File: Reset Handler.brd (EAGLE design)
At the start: 67 x 39.4 mm, 13 parts, among them IC1 NE555P, T1 2N222A

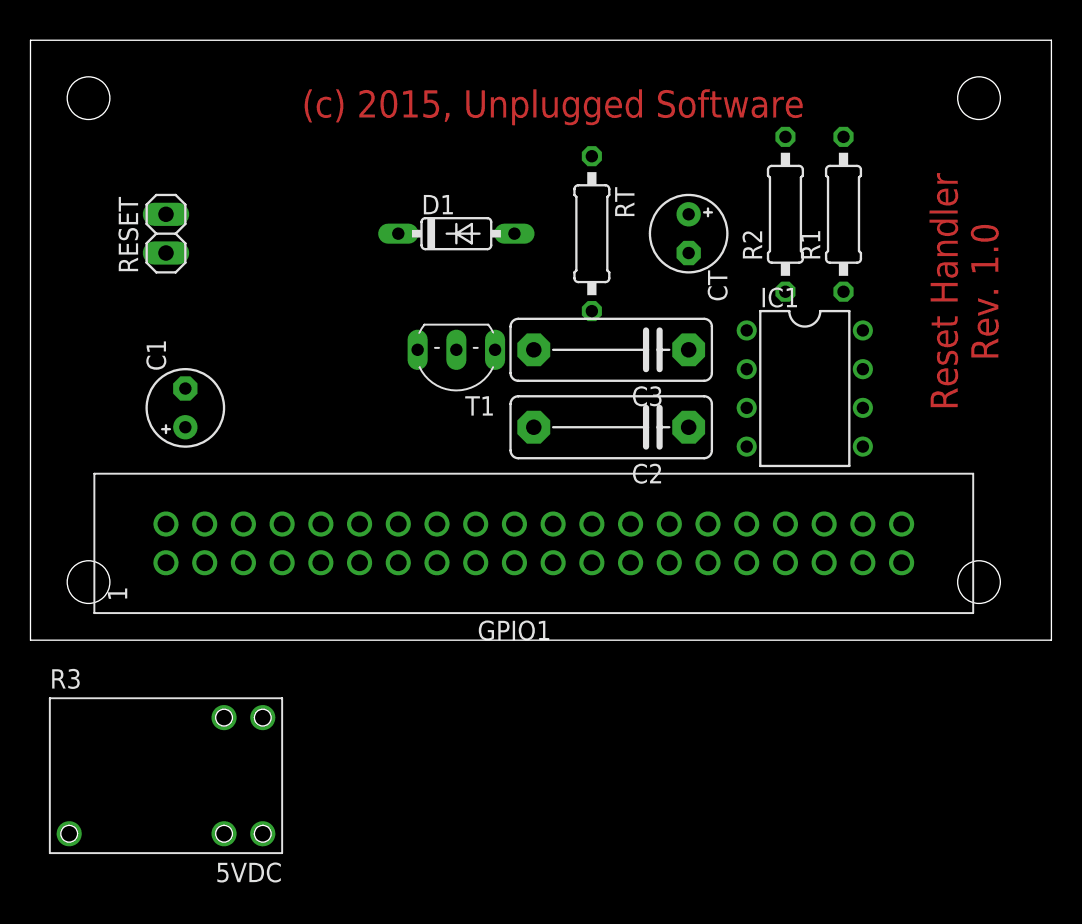
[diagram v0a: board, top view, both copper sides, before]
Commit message: Finished Reset Handler board.
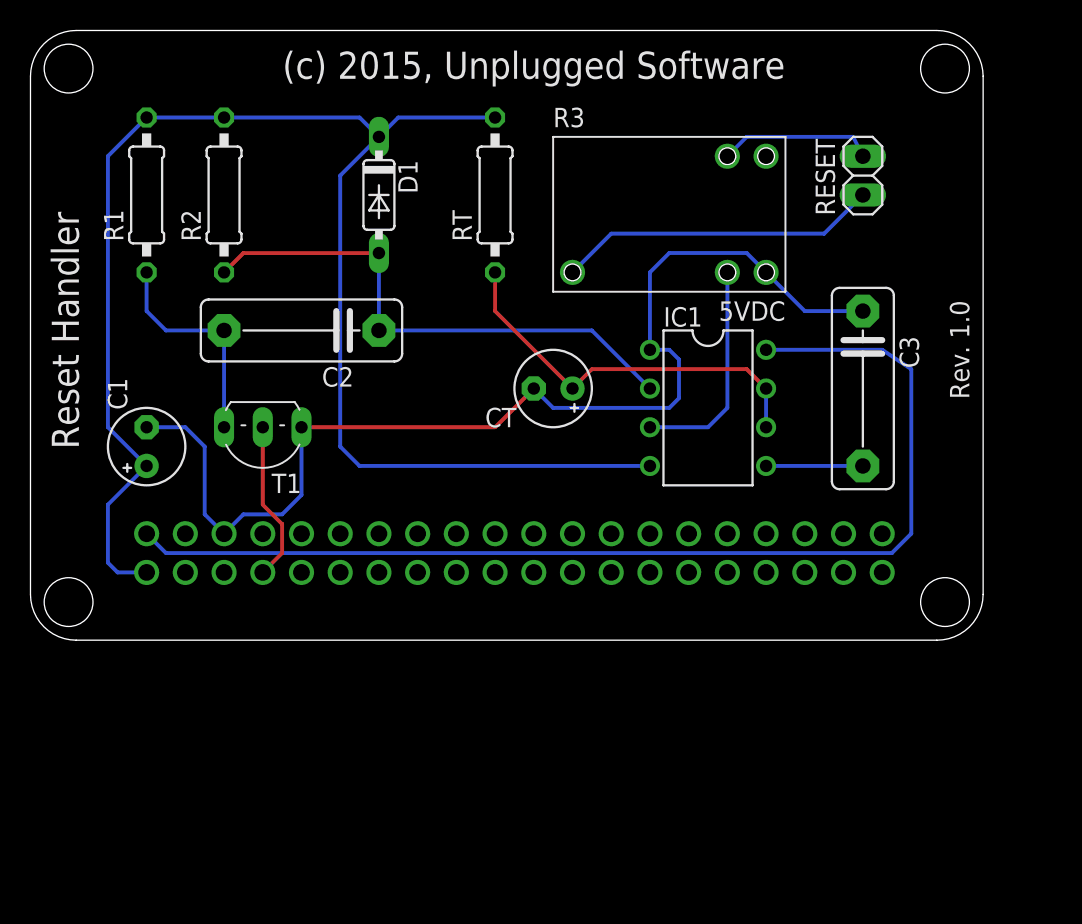
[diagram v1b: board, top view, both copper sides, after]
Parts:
- D1: value 1N4148DO35-7 -> 1N4148
- GPIO1: value RPI_GPIOUPPER -> RPI_GPIO_MALE_OPEN; device connectors:RPI_GPIO_MALE -> connectors:RPI_GPIO_FEMALE_TOP
- moved R3 49.5 mm to (41.9, 27.9)
- moved RESET 45.9 mm to (54.6, 30.5)
- moved R1 45.7 mm to (7.62, 29.2)
- moved R2 36.9 mm to (12.7, 29.2)
- moved C2 21.3 mm to (17.8, 20.3)
- moved C3 16.7 mm to (54.6, 16.5), turned to 270 degrees
- moved T1 13.7 mm to (15.2, 12.7)
- moved CT 13.5 mm to (34.3, 16.5), turned to 180 degrees
- moved RT 6.84 mm to (30.5, 29.2), turned to 90 degrees
- moved IC1 6.48 mm to (44.5, 15.2)
- moved D1 5.68 mm to (22.9, 29.2), turned to 270 degrees
- moved C1 3.59 mm to (7.62, 12.7)
- moved GPIO1 0.63 mm to (31.8, 5.71)
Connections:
- new net N$5: C3.2, IC1.5
- net GND: no longer C3.2, IC1.5
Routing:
- net +3.3VDC: track 0.00 -> 101.3 mm
- net GND: track 0.00 -> 73.6 mm
- net N$4: track 0.00 -> 71.9 mm
- net N$2: track 0.00 -> 35.1 mm
- net N$3: track 0.00 -> 26.0 mm
- net N$6: track 0.00 -> 21.2 mm
- net RESET_OUT: track 0.00 -> 14.5 mm
- net N$1: track 0.00 -> 14.5 mm
- net GPIO_4: track 0.00 -> 10.6 mm
- net N$7: track 0.00 -> 10.2 mm
- net N$5: track 0.00 -> 6.35 mm
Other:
- board size 67 x 39.4 mm -> 62.5 x 40 mm
- board text added: "Reset Handler"
- board text added: "Rev. 1.0"
- board text removed: "Reset Handler Rev. 1.0"
